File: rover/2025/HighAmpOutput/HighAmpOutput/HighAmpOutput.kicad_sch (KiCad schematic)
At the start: 14 parts, among them J1 JST3_Pin, U1 HSS-VN7004SLHTR, U10 XT60PM-F, U2 XT60PM-F, U3 XT60-F, U4 XT60-F, U5 XT60-F, U6 XT60-F, U7 XT60-F, U8 XT60-F, U9 XT60PM-F

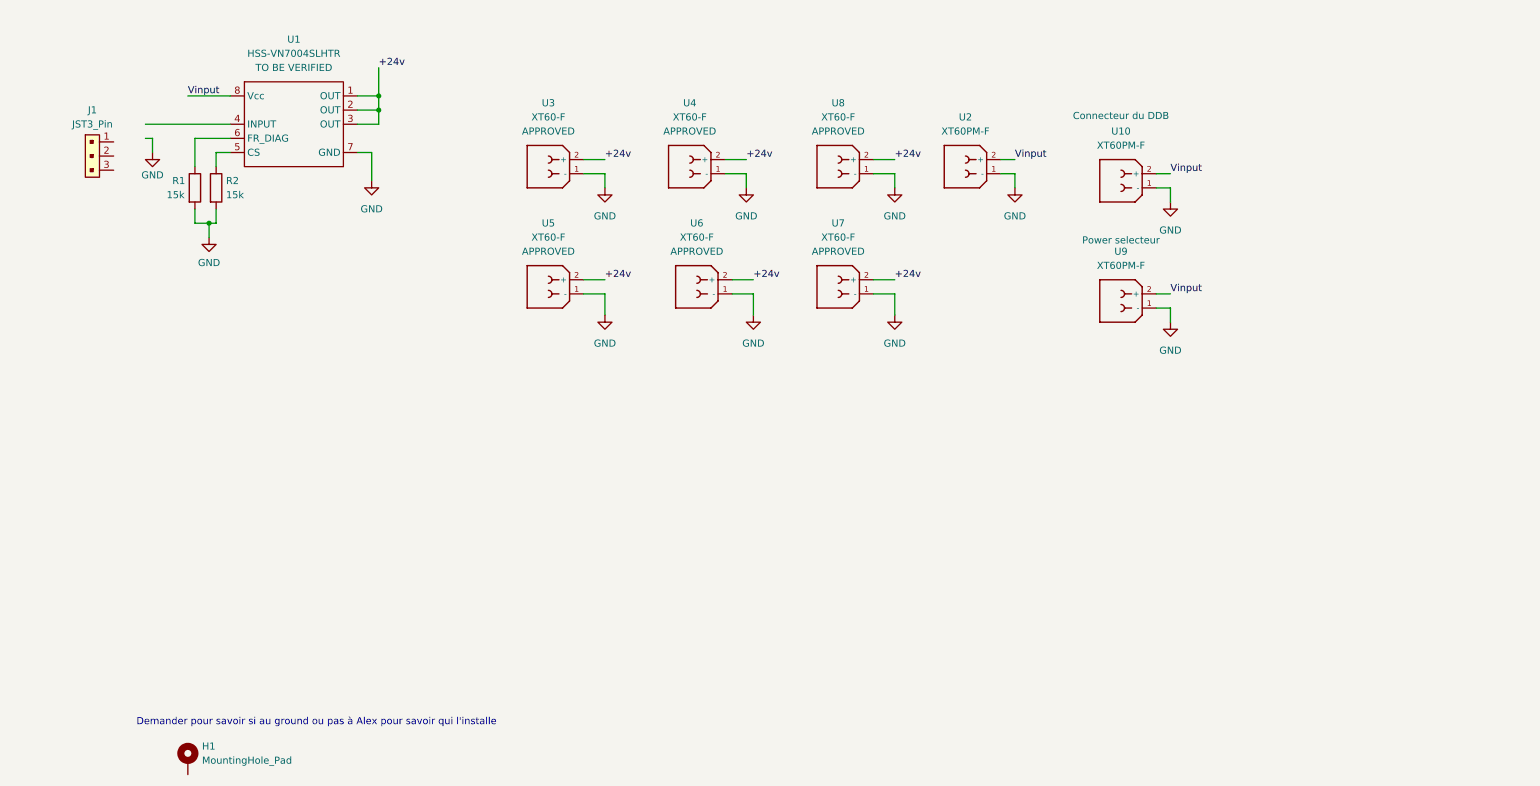
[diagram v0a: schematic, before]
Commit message: Update_HighAmpOut_2025-02-08
Avancement de la shématique
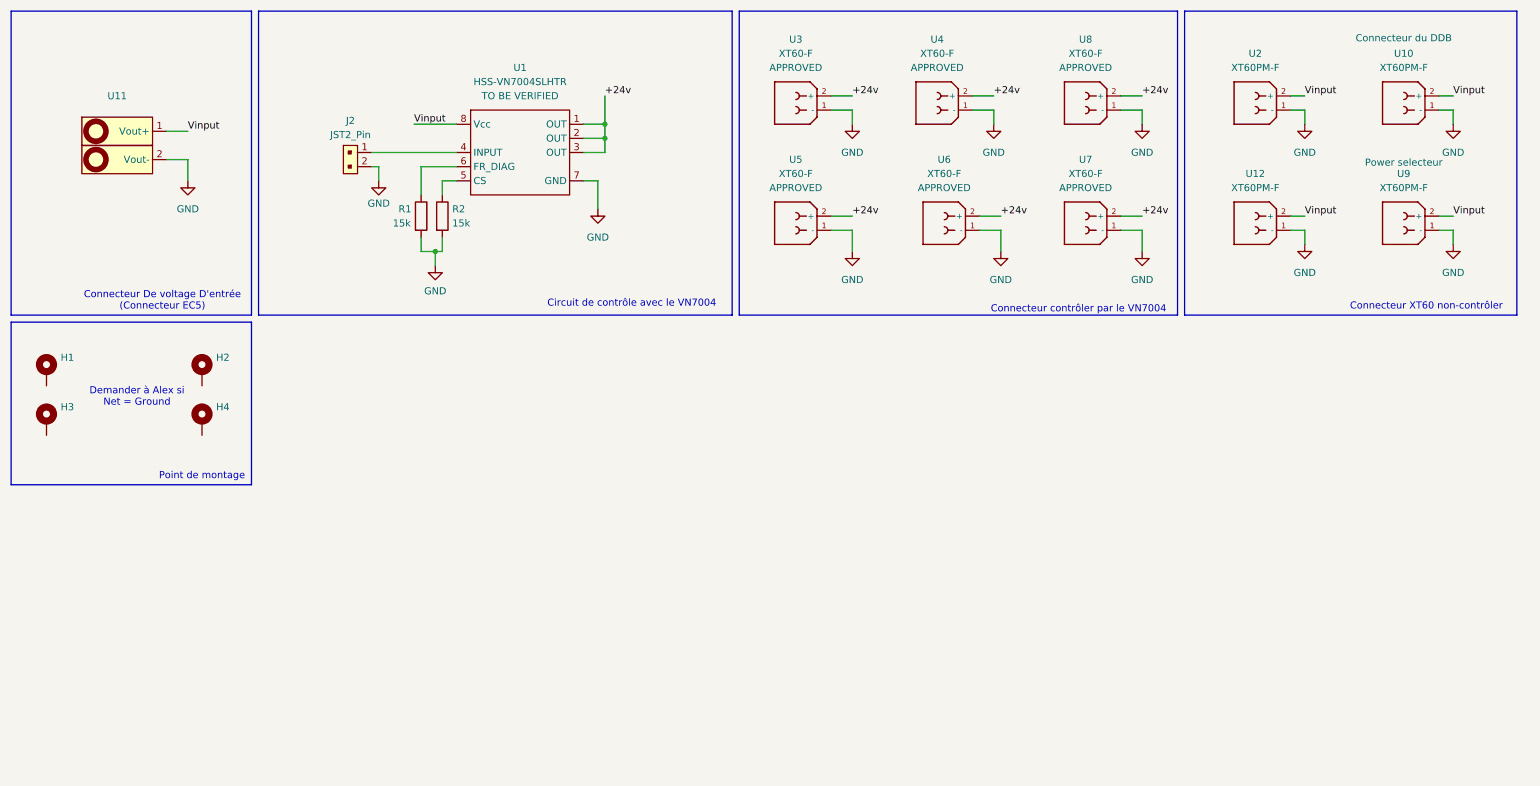
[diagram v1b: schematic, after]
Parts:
- removed J1: JST3_Pin, Connector_JST:JST_XH_B3B-XH-AM_1x03_P2.50mm_Vertical, symbol RoverLibrary:CONN-JST-XH-B3B
- added H2, H3, H4: MountingHole_Pad, MountingHole:MountingHole_3.2mm_M3_DIN965_Pad_TopBottom, symbol RoverLibrary:MountingHole_Pad
- added J2: JST2_Pin, RoverFootprint:2-pins-JST_XH_B2B-XH-A_1x02_P2.50mm_Vertical, symbol RoverLibrary:CONN-JST-XH-B2B
- added U11: ~, RoverFootprint:EC5, symbol RoverLibrary:EC5
- added U12: XT60PM-F, RoverFootprint:AMASS_XT60PW-F_1x02_P7.20mm_Horizontal, symbol RoverLibrary:XT60PW-F
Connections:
- net GND: now also J2.2, U11.2 (Vout-), U12.1 (-)
- net Vinput: now also U11.1 (Vout+), U12.2 (+)
- net at U1.4 (INPUT): now also J2.1
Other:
- note added: "Circuit de contrôle avec le VN7004"
- note added: "Connecteur De voltage D'entrée (Connecteur EC5)"
- note added: "Connecteur XT60 non-contrôler"
- note added: "Connecteur contrôler par le VN7004"
- note added: "Demander à Alex si Net = Ground"
- note added: "Point de montage"
- note removed: "Demander pour savoir si au ground ou pas à Alex pour savoir qui l'installe"
- moved on the sheet: H1, R1, R2, U1, U10, U2, U3, U4, U5, U6, U7, U8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
